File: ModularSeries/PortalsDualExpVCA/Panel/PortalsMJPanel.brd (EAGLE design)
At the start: 48.5 x 100 mm, 12 parts

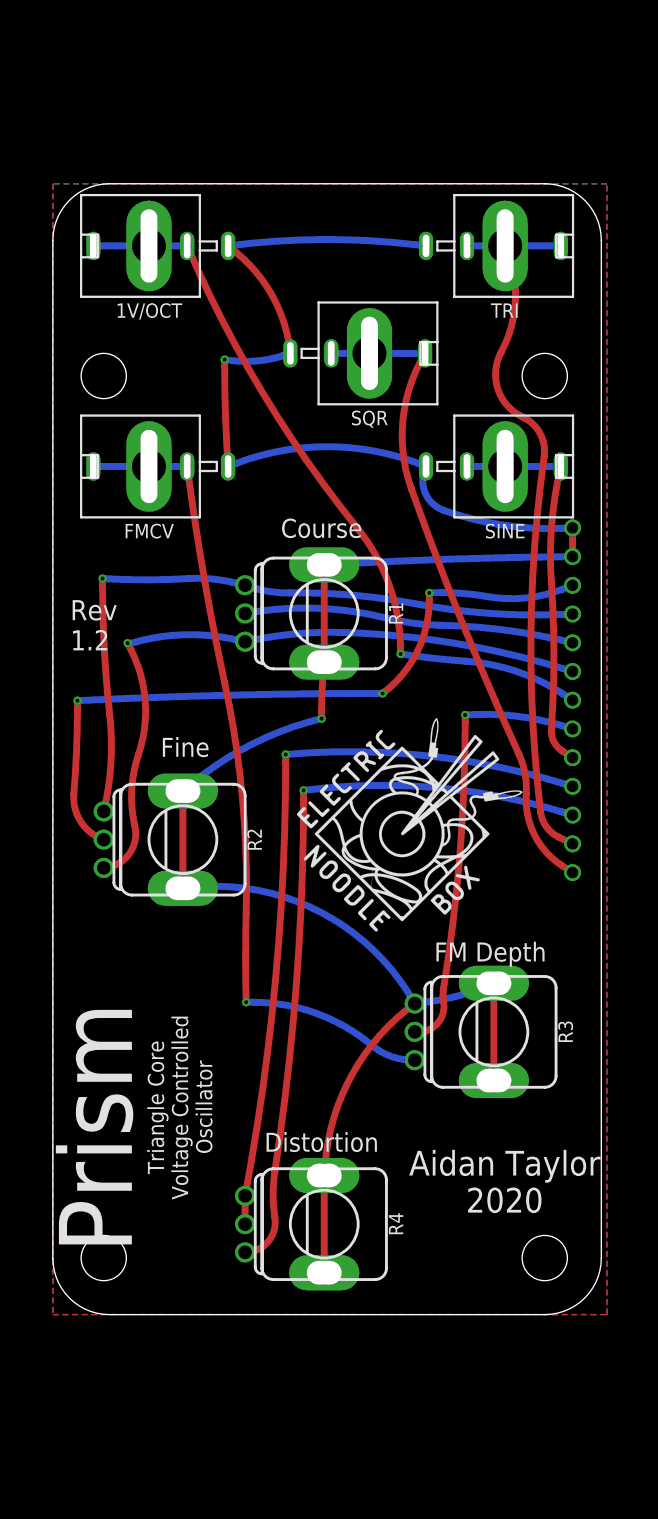
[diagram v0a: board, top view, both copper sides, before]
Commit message: Fields added and various updates to designs
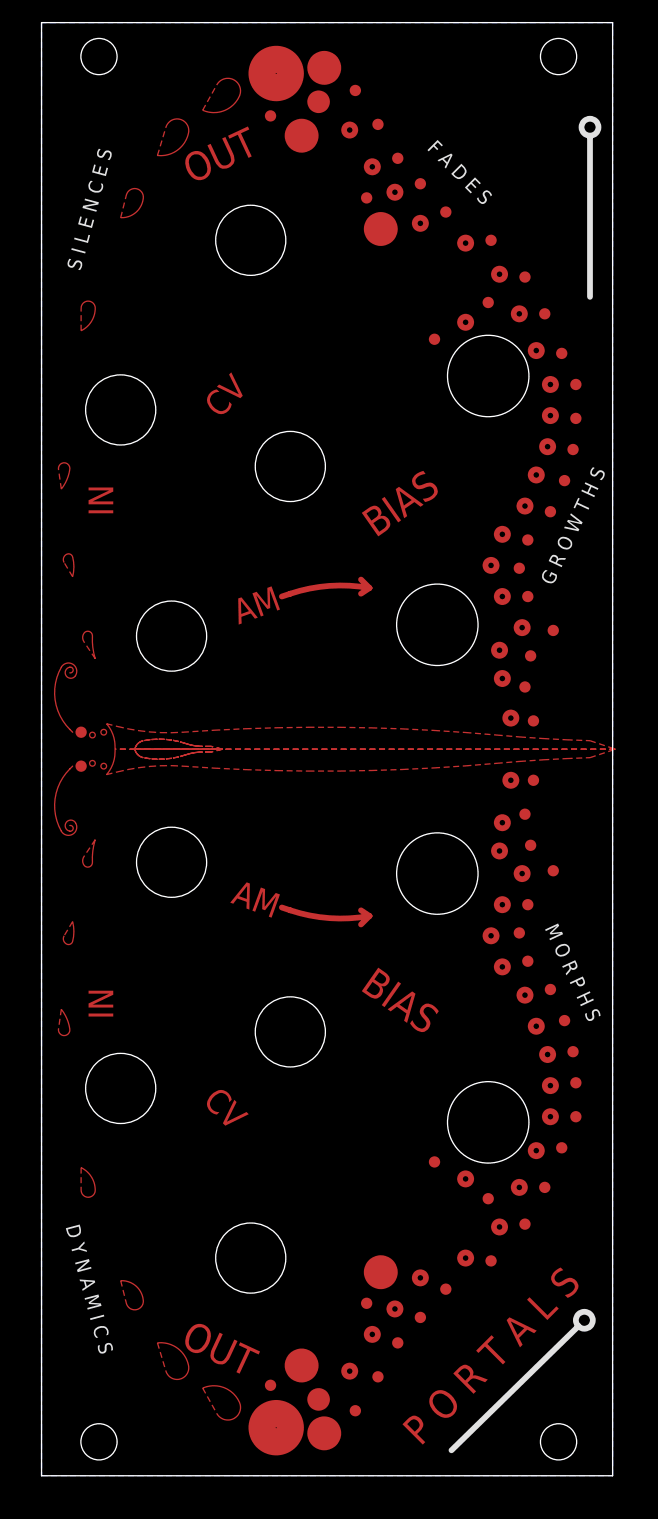
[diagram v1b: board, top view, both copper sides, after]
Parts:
- removed 1V/OCT, FMCV, SINE, SQR, TRI: COMBI-JACKCINCHNANA, ElectricNoodleBox:NEWCOMBOJACK_PANEL
- removed BOARD1: PRISM_LINK, ElectricNoodleBox:PRISM
- removed R1, R2, R3, R4: B100K, ElectricNoodleBox:ALPHA_RV09_9MMPOT
- removed U$1, U$2: (no value), ElectricNoodleBox:LOGO20X20
- added E$11, E$12, E$13, E$14: (no value), ElectricNoodleBox:ALPHA9MM_POT_CUTOUT
- added E$15: (no value), ElectricNoodleBox:LOGO20X20
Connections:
- removed net AGND: 1V/OCT.S, BOARD1.GNDA, BOARD1.GNDB, FMCV.S, R1.LUGL, R1.LUGR, R2.LUGL, R2.LUGR, R3.C1, R3.LUGL, R3.LUGR, R4.LUGL, R4.LUGR, SINE.S, SQR.S, TRI.S
- removed net N$1: 1V/OCT.CONN, 1V/OCT.T1, 1V/OCT.T2, BOARD1.CVA
- removed net N$10: BOARD1.SIN, SINE.CONN, SINE.T1, SINE.T2
- removed net N$11: BOARD1.TRI, TRI.CONN, TRI.T1, TRI.T2
- removed net N$12: BOARD1.SQR, SQR.CONN, SQR.T1, SQR.T2
- removed net N$2: BOARD1.F1, R1.C1, R2.C1
- removed net N$3: BOARD1.F3, R1.C3, R2.C3
- removed net N$4: BOARD1.F2, R1.C2
- removed net N$5: BOARD1.FINE, R2.C2
- removed net N$6: FMCV.CONN, FMCV.T1, FMCV.T2, R3.C3
- removed net N$7: BOARD1.CVB, R3.C2
- removed net N$8: BOARD1.DIST1, R4.C1, R4.C2
- removed net N$9: BOARD1.DIST2, R4.C3
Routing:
- net AGND: track 202.4 -> 0.00 mm, vias 2 -> 0
- net N$6: track 71.8 -> 0.00 mm, vias 1 -> 0
- net N$8: track 67.2 -> 0.00 mm, vias 1 -> 0
- net N$9: track 65.8 -> 0.00 mm, vias 1 -> 0
- net N$1: track 65.1 -> 0.00 mm, vias 1 -> 0
- net N$11: track 63.3 -> 0.00 mm
- net N$5: track 62.7 -> 0.00 mm, vias 3 -> 0
- net N$2: track 62.4 -> 0.00 mm, vias 1 -> 0
- net N$3: track 60.6 -> 0.00 mm, vias 1 -> 0
- net N$12: track 57.4 -> 0.00 mm
- net N$7: track 38.7 -> 0.00 mm, vias 1 -> 0
- net N$10: track 34.8 -> 0.00 mm
- net N$4: track 29.1 -> 0.00 mm
- net S$30: track 0.00 -> 7.02 mm
- net S$26: track 0.00 -> 7.02 mm
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- added copper zone on layer 1, net BODY
- added copper zone on layer 1, net BODY1
- added copper zone on layer 1, net CREST4
- added copper zone on layer 1, net CREST5
- added copper zone on layer 1, net CREST6
- added copper zone on layer 1, net CREST7
- added copper zone on layer 16, net GND
- added copper zone on layer 1, net S$1
- added copper zone on layer 1, net S$18
- added copper zone on layer 1, net S$19
- added copper zone on layer 1, net S$2
- added copper zone on layer 1, net S$20
- added copper zone on layer 1, net S$21
- added copper zone on layer 1, net S$22
- added copper zone on layer 1, net S$23
- added copper zone on layer 1, net S$24
- added copper zone on layer 1, net S$3
- added copper zone on layer 1, net S$4
- added copper zone on layer 1, net S$5
- added copper zone on layer 1, net S$6
- added copper zone on layer 1, net S$7
- removed copper zone on layer 1, net AGND
- removed copper zone on layer 16, net AGND
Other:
- board size 48.5 x 100 mm -> 50.5 x 128.5 mm
- board text added: "AM"
- board text added: "BIAS"
- board text added: "CV"
- board text added: "D Y N A M I C S"
- board text added: "F A D E S"
- board text added: "G R O W T H S"
- board text added: "IN"
- board text added: "M O R P H S"
- board text added: "OUT"
- board text added: "P O R T A L S"
- board text added: "S I L E N C E S"
- board text removed: "Aidan Taylor 2020"
- board text removed: "Course"
- board text removed: "Distortion"
- board text removed: "FM Depth"
- board text removed: "Fine"
- board text removed: "Prism"
- board text removed: "Rev 1.2"
- board text removed: "Triangle Core Voltage Controlled Oscillator"
